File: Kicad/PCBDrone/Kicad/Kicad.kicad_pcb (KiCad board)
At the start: 4 copper layers, 130 x 130 mm, 90 parts, among them J1 Conn_01x02_Pin, J2 Conn_01x04, U1 ESP32-WROOM-32E, U2 BMI323, U3 DRV8210DSGR, U4 DRV8210DSGR, U5 DRV8210DSGR, U6 DRV8210DSGR

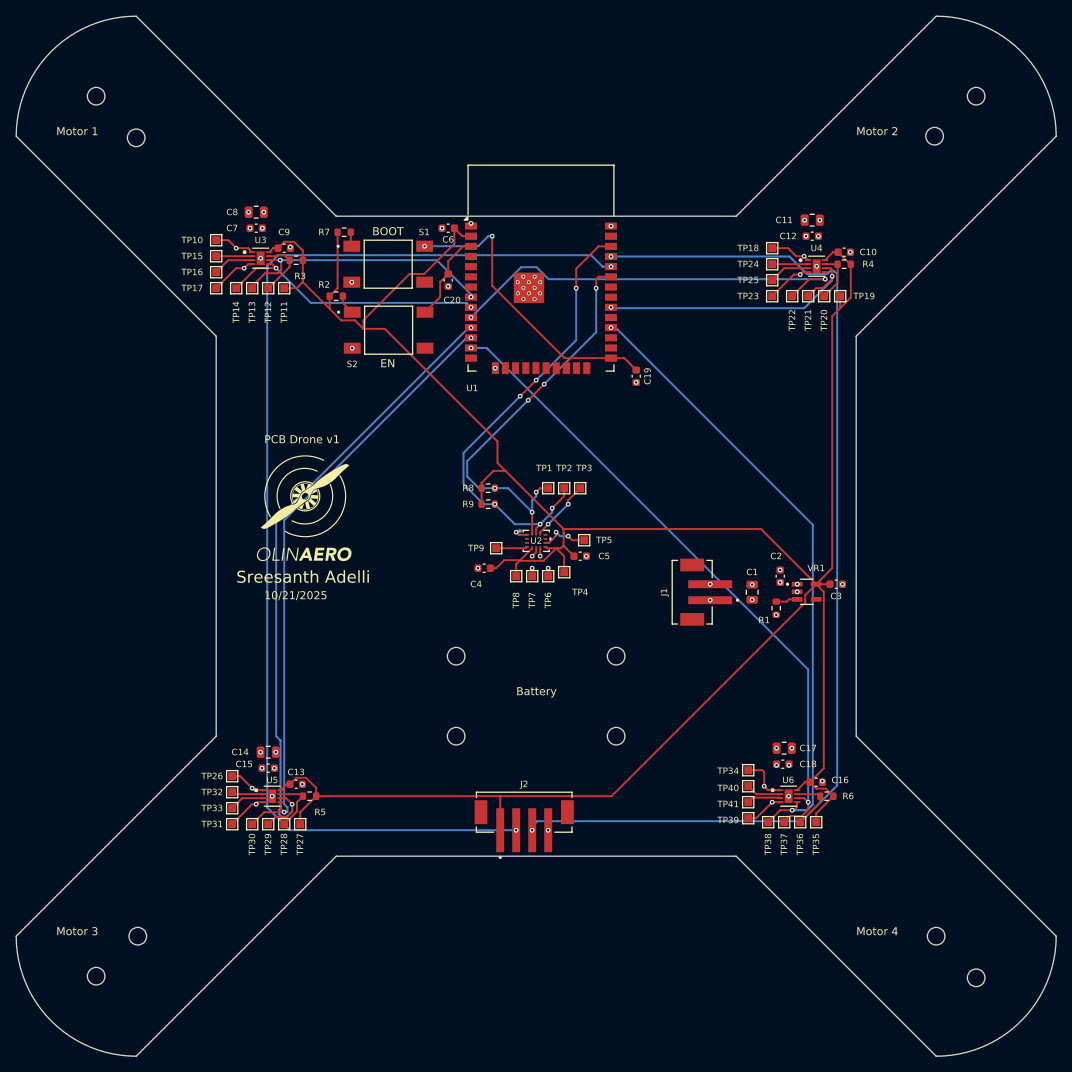
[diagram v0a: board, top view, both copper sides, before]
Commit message: hi
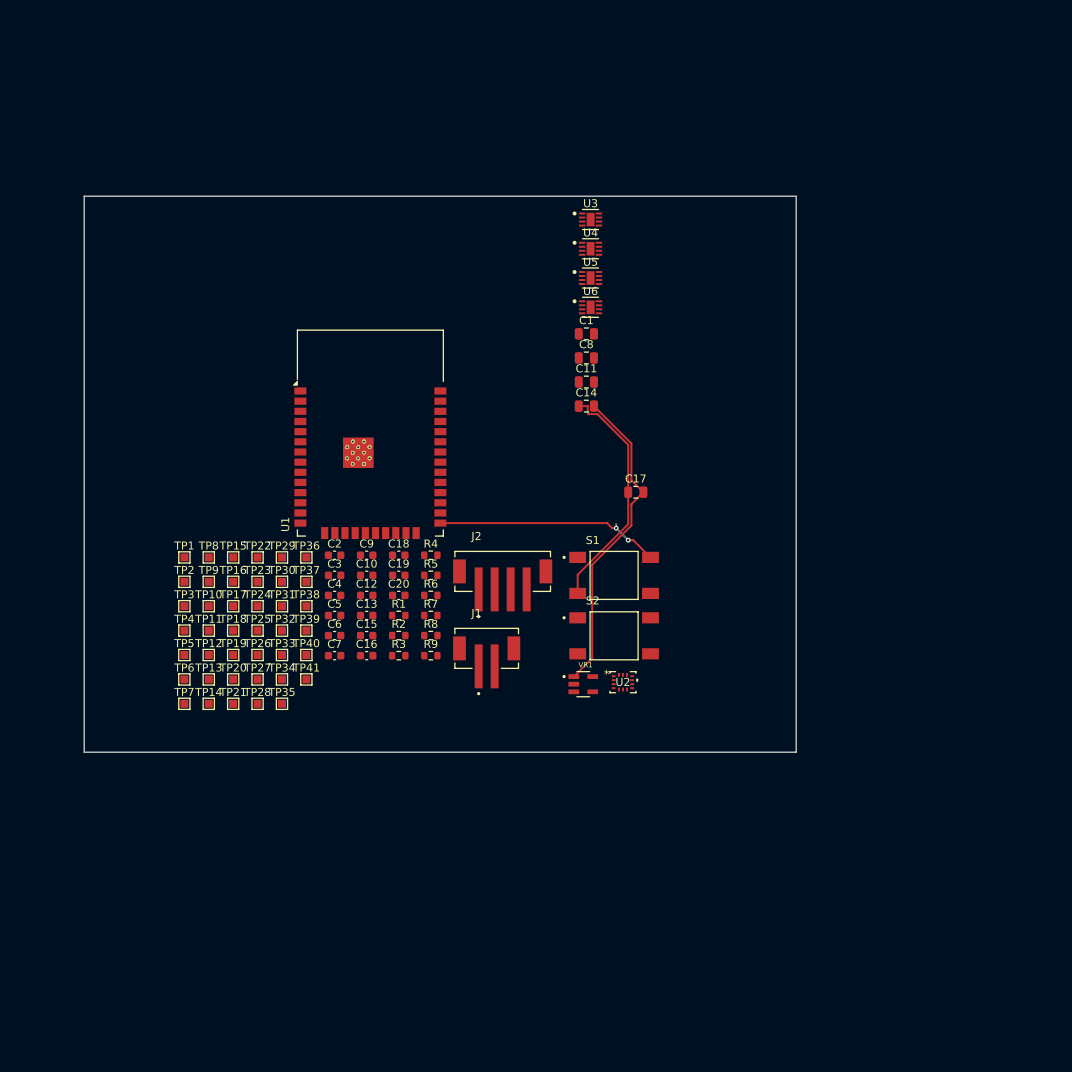
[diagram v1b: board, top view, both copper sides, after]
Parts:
- removed G***: LOGO, footprints:Logo
- removed Motor Mount: Motor Mount, MountingHole:MotorMount (x4)
- removed REF** (x4): MountingHole_2.2mm_M2, MountingHole:MountingHole_2.2mm_M2
- moved TP19 88.1 mm to (112.1, 114.9)
- moved TP21 88.1 mm to (112.1, 121.0)
- moved TP20 88.0 mm to (112.1, 117.9)
- moved TP18 82.6 mm to (112.1, 111.8)
- moved TP25 77.8 mm to (115.2, 111.8)
- moved TP24 77.2 mm to (115.2, 108.8)
- moved U5 76.0 mm to (156.8, 67.7)
- moved TP22 74.4 mm to (115.2, 102.7)
- moved TP23 73.6 mm to (115.2, 105.7)
- moved C10 72.1 mm to (128.8, 104.9)
- moved C12 71.5 mm to (128.8, 107.4), turned to 0 degrees
- moved TP36 70.0 mm to (121.3, 102.7)
- moved TP35 68.4 mm to (118.2, 121.0)
- moved TP37 66.9 mm to (121.3, 105.7)
- moved U6 65.9 mm to (156.8, 71.4)
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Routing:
- net /VCC_3V3: track 328.9 -> 0.00 mm
- net /ESP_UART_RX: track 144.1 -> 0.00 mm, vias 2 -> 0
- net /ESP_UART_TX: track 134.1 -> 0.00 mm, vias 2 -> 0
- net /MOTOR4_INPUT1: track 81.6 -> 0.00 mm, vias 2 -> 0
- net /MOTOR4_INPUT2: track 81.2 -> 0.00 mm, vias 2 -> 0
- net /MOTOR3_INPUT1: track 80.8 -> 0.00 mm, vias 2 -> 0
- net /MOTOR3_INPUT2: track 75.9 -> 0.00 mm, vias 2 -> 0
- net /SCL: track 57.0 -> 0.00 mm, vias 6 -> 0
- net /MOTOR2_INPUT2: track 53.4 -> 0.00 mm, vias 2 -> 0
- net /SDA: track 50.4 -> 0.00 mm, vias 6 -> 0
- net /MOTOR2_INPUT1: track 35.6 -> 0.00 mm, vias 2 -> 0
- net /MOTOR1_INPUT1: track 33.7 -> 0.00 mm, vias 2 -> 0
- net /MOTOR1_INPUT2: track 33.5 -> 0.00 mm, vias 2 -> 0
- net /VBAT: track 21.0 -> 40.0 mm, vias 17 -> 0
- net Net-(U1-EN): track 11.2 -> 0.00 mm
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- added copper zone on In2.Cu, net /VCC_3V3
- removed copper zone on In2.Cu, net /VBAT
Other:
- board size 130 x 130 mm -> 89 x 69.5 mm
- board text removed: "10/21/2025"
- board text removed: "BOOT"
- board text removed: "Battery"
- board text removed: "EN"
- board text removed: "Motor 1"
- board text removed: "Motor 2"
- board text removed: "Motor 3"
- board text removed: "Motor 4"
- board text removed: "PCB Drone v1"
- board text removed: "Sreesanth Adelli"
